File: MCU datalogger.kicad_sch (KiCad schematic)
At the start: 25 parts, among them U1 24LC1025, U2 24LC1025, U3 DS1337S_, U4 ATMEGA328P-AU, Y1 16 MHz, Y2 32.768 KHz

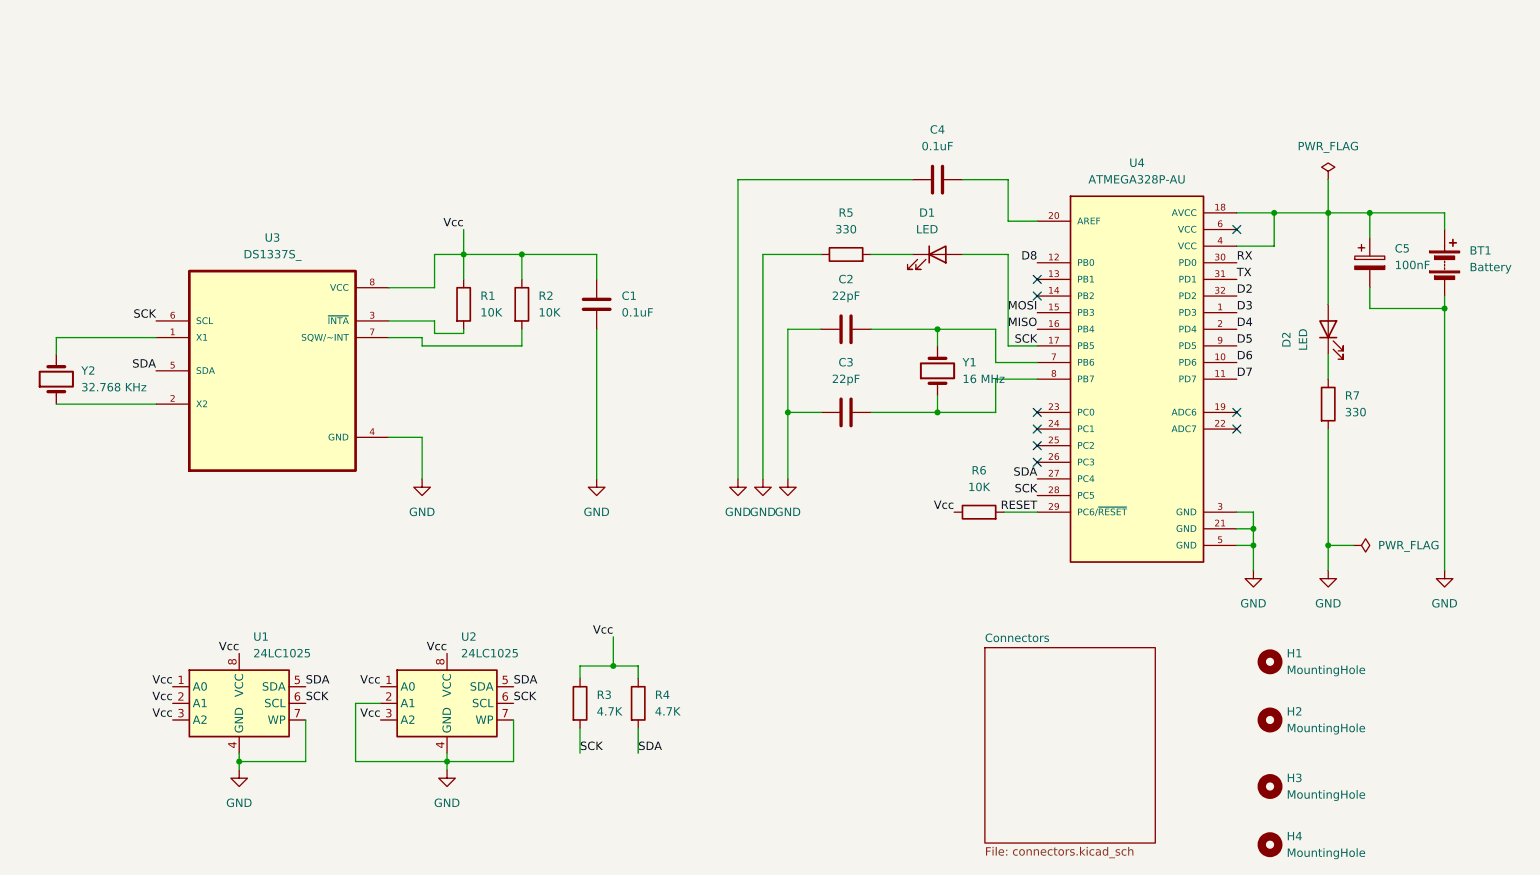
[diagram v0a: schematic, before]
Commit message: changes in both sheets
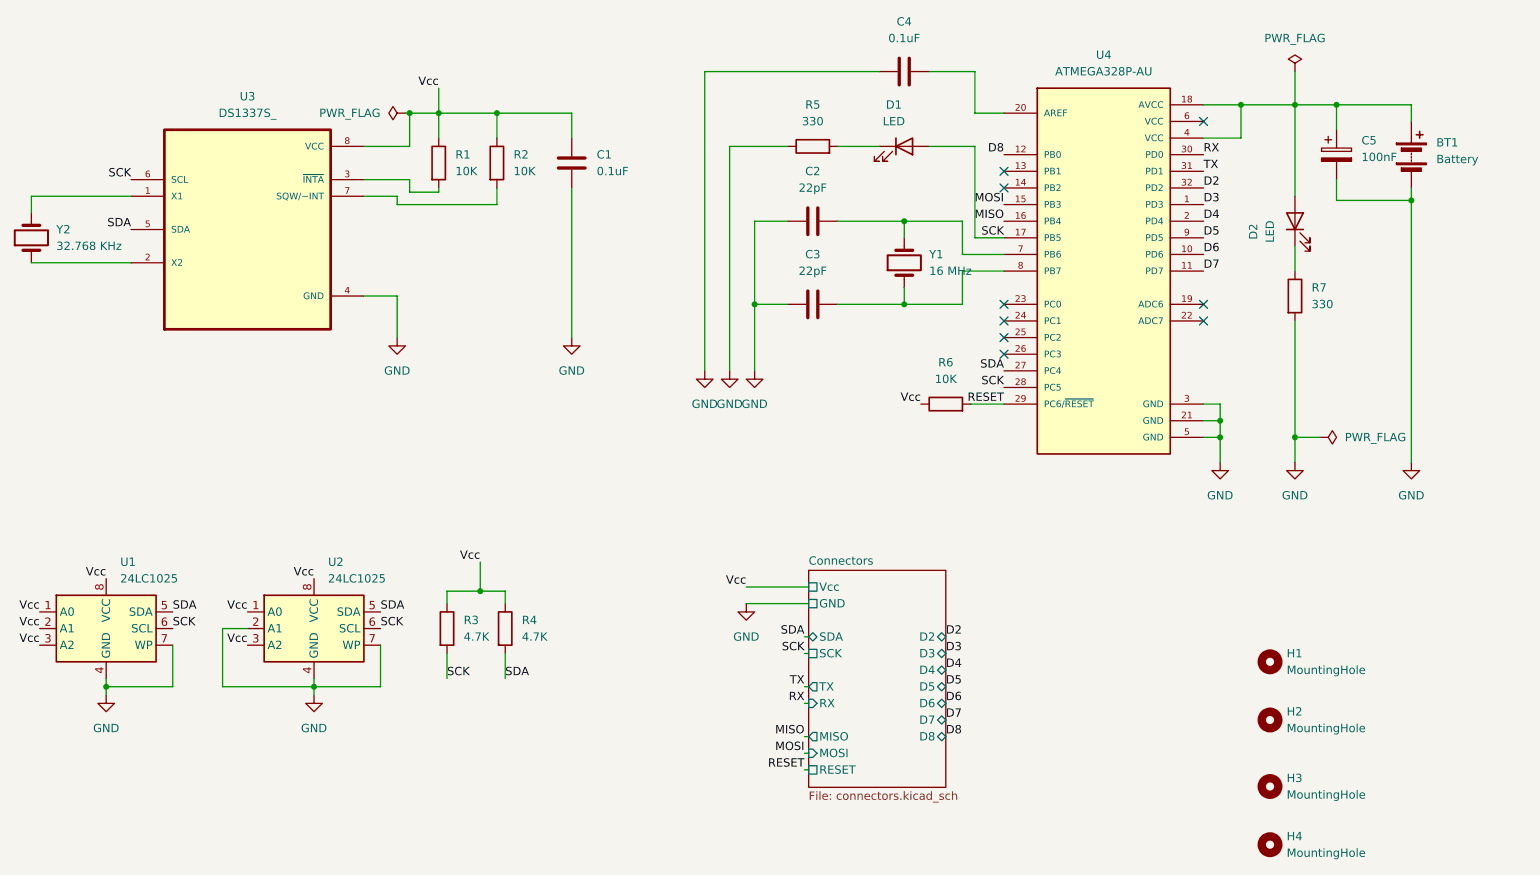
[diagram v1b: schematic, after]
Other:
- sheet Connectors ports: added D2, D3, D4, D5, D6, D7, D8, GND, MISO, MOSI, RESET, RX, SCK, SDA, TX, Vcc; removed none
- moved on the sheet: BT1, C1, C2, C3, C4, C5, D1, D2, R1, R2, R3, R4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
